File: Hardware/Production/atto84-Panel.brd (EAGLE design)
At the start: 101.1 x 104.9 mm, 1062 parts, among them U1 ATTINY84ATTINY84-20MU, U10 ATTINY84ATTINY84-20MU, U11 ATTINY84ATTINY84-20MU, U12 ATTINY84ATTINY84-20MU, U13 ATTINY84ATTINY84-20MU, U14 ATTINY84ATTINY84-20MU, U15 ATTINY84ATTINY84-20MU, U16 ATTINY84ATTINY84-20MU, U17 ATTINY84ATTINY84-20MU, U18 ATTINY84ATTINY84-20MU, U19 ATTINY84ATTINY84-20MU, U2 ATTINY84ATTINY84-20MU, U20 ATTINY84ATTINY84-20MU, U21 ATTINY84ATTINY84-20MU, U22 ATTINY84ATTINY84-20MU, U23 ATTINY84ATTINY84-20MU, U24 ATTINY84ATTINY84-20MU, U3 ATTINY84ATTINY84-20MU, U4 ATTINY84ATTINY84-20MU, U5 ATTINY84ATTINY84-20MU, U6 ATTINY84ATTINY84-20MU, U7 ATTINY84ATTINY84-20MU, U8 ATTINY84ATTINY84-20MU, U9 ATTINY84ATTINY84-20MU

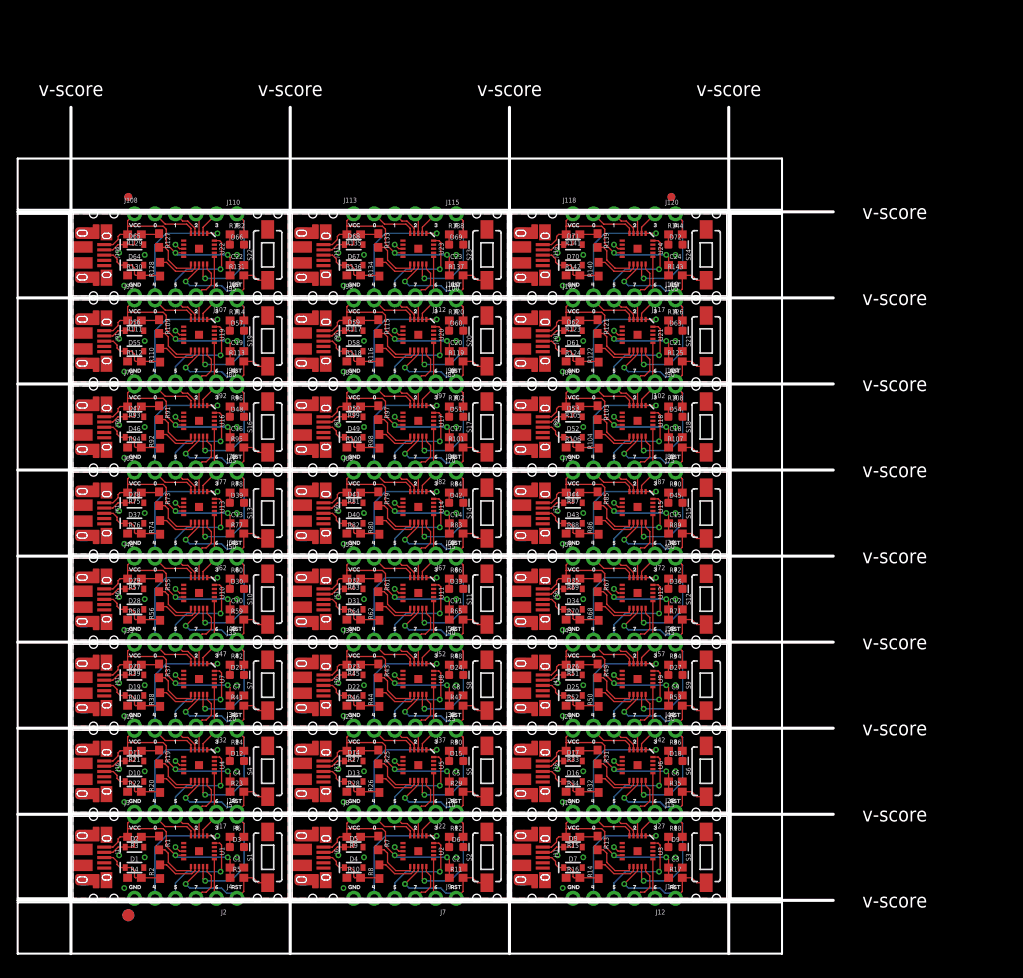
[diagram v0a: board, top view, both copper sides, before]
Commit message: Pushing "new" version
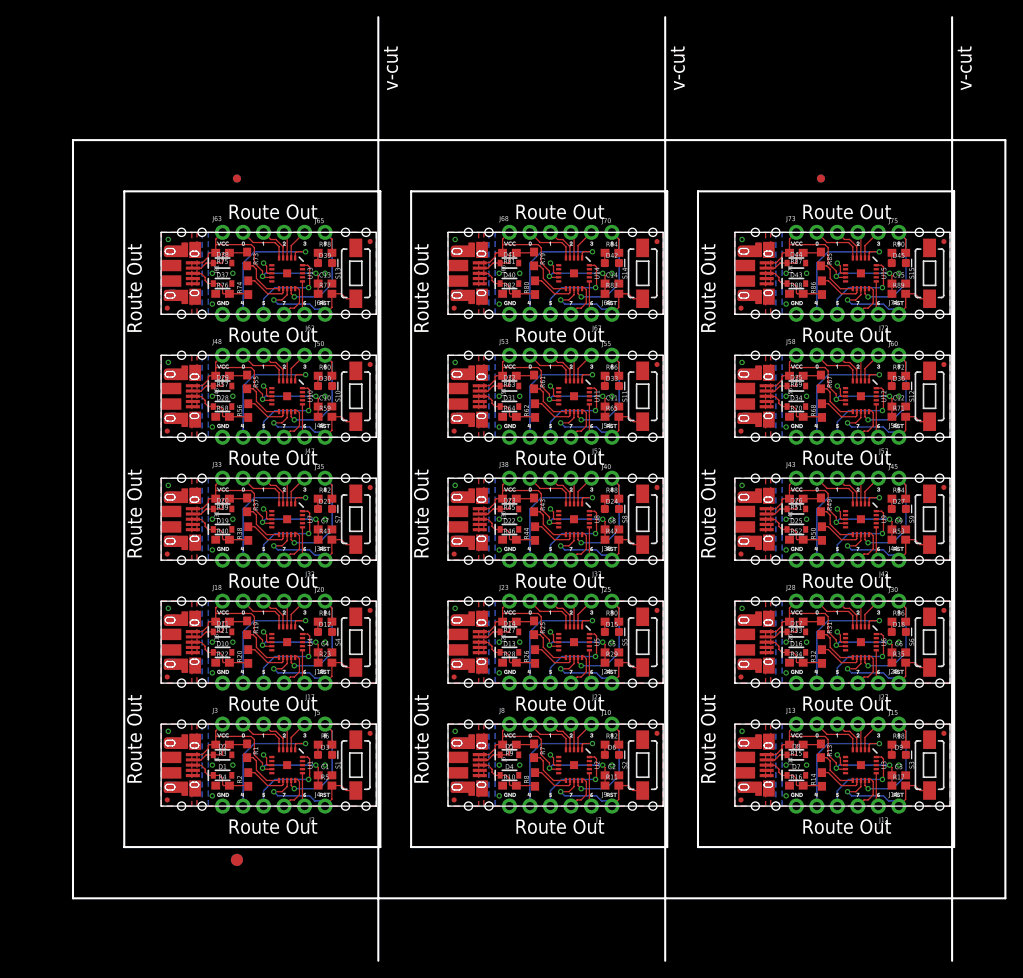
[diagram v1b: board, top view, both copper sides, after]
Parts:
- removed C16, C17, C18, C19, C20, C21, C22, C23, C24: 0.1uF, SparkFun-Capacitors:0603
- removed D46, D47, D49, D50, D52, D53, D55, D56, D58, D59, D61, D62, D64, D65, D67, D68, D70, D71: 3.6V, SparkFun-DiscreteSemi:SOD-323
- removed D48, D51, D54, D57, D60, D63, D66, D69, D72: BLUE, SparkFun-LED:LED-0603
- removed J100, J104, J105, J109, J110, J114, J115, J119, J120, J79, J80, J84, J85, J89, J90, J94, J95, J99: (no value), SparkFun-Connectors:1X01_NO_SILK
- removed J101, J106, J111, J116, J76, J81, J86, J91, J96: (no value), SparkFun-Connectors:USB-MICROB-PTH-MILL
- removed J102, J103, J107, J108, J112, J113, J117, J118, J77, J78, J82, J83, J87, J88, J92, J93, J97, J98: (no value), SparkFun-Connectors:1X05_NO_SILK
- removed R100, R106, R112, R118, R124, R130, R136, R142, R94: 1M, SparkFun-Resistors:0603
- removed R101, R107, R113, R119, R125, R131, R137, R143, R95: 10k, SparkFun-Resistors:0603
- removed R102, R108, R114, R120, R126, R132, R138, R144, R96: 1k, SparkFun-Resistors:0603
- removed R103, R104, R109, R110, R115, R116, R121, R122, R127, R128, R133, R134, R139, R140, R91, R92, R97, R98: 68OHM-0603-1/10W-1%, SparkFun-Resistors:0603
- removed R105, R111, R117, R123, R129, R135, R141, R93, R99: 1.5k, SparkFun-Resistors:0603
- removed S16, S17, S18, S19, S20, S21, S22, S23, S24: MOMENTARY-SWITCH-SPST-SMD-6.0X3.5MM, SparkFun-Switches:TACTILE_SWITCH_SMD_6.0X3.5MM
- removed U$406, U$433, U$460, U$487, U$514, U$541, U$568, U$595, U$622: (no value), buzzard_labels (20):00
- removed U$407, U$434, U$461, U$488, U$515, U$542, U$569, U$596, U$623: (no value), buzzard_labels (20):11
- removed U$408, U$435, U$462, U$489, U$516, U$543, U$570, U$597, U$624: (no value), buzzard_labels (20):22
- removed U$409, U$436, U$463, U$490, U$517, U$544, U$571, U$598, U$625: (no value), buzzard_labels (20):33
- removed U$410, U$437, U$464, U$491, U$518, U$545, U$572, U$599, U$626: (no value), buzzard_labels (20):44
- removed U$411, U$438, U$465, U$492, U$519, U$546, U$573, U$600, U$627: (no value), buzzard_labels (20):55
- removed U$412, U$439, U$466, U$493, U$520, U$547, U$574, U$601, U$628: (no value), buzzard_labels (20):66
- removed U$413, U$440, U$467, U$494, U$521, U$548, U$575, U$602, U$629: (no value), buzzard_labels (20):77
- removed U$414, U$441, U$468, U$495, U$522, U$549, U$576, U$603, U$630: (no value), buzzard_labels (20):RST8
- removed U$415, U$442, U$469, U$496, U$523, U$550, U$577, U$604, U$631: (no value), buzzard_labels (20):VCC10
- removed U$416, U$443, U$470, U$497, U$524, U$551, U$578, U$605, U$632: (no value), buzzard_labels (20):GND9
- removed U$417, U$444, U$471, U$498, U$525, U$552, U$579, U$606, U$633: (no value), buzzard_labels (21):81
- removed U$418, U$445, U$472, U$499, U$526, U$553, U$580, U$607, U$634: (no value), buzzard_labels (20):ATTO8411
- removed U$419, U$446, U$473, U$500, U$527, U$554, U$581, U$608, U$635: (no value), SparkX:SPARKX-SMALL
- removed U$420, U$447, U$474, U$501, U$528, U$555, U$582, U$609, U$636: (no value), buzzard_labels (22):VCC_5
- removed U$421, U$448, U$475, U$502, U$529, U$556, U$583, U$610, U$637: (no value), buzzard_labels (22):0_4
- removed U$422, U$449, U$476, U$503, U$530, U$557, U$584, U$611, U$638: (no value), buzzard_labels (22):1_3
- removed U$423, U$450, U$477, U$504, U$531, U$558, U$585, U$612, U$639: (no value), buzzard_labels (22):2_2
- removed U$424, U$451, U$478, U$505, U$532, U$559, U$586, U$613, U$640: (no value), buzzard_labels (22):3_1
- removed U$425, U$452, U$479, U$506, U$533, U$560, U$587, U$614, U$641: (no value), buzzard_labels (22):8_0
- removed U$426, U$453, U$480, U$507, U$534, U$561, U$588, U$615, U$642: (no value), SparkFun-Aesthetics:OSHW-LOGO-S
- removed U$427, U$454, U$481, U$508, U$535, U$562, U$589, U$616, U$643: (no value), buzzard_labels (23):_#RST0
- removed U$428, U$455, U$482, U$509, U$536, U$563, U$590, U$617, U$644: (no value), buzzard_labels (23):_42
- removed U$429, U$456, U$483, U$510, U$537, U$564, U$591, U$618, U$645: (no value), buzzard_labels (23):_53
- removed U$430, U$457, U$484, U$511, U$538, U$565, U$592, U$619, U$646: (no value), buzzard_labels (23):_64
- removed U$431, U$458, U$485, U$512, U$539, U$566, U$593, U$620, U$647: (no value), buzzard_labels (23):_75
- removed U$432, U$459, U$486, U$513, U$540, U$567, U$594, U$621, U$648: (no value), buzzard_labels (23):_GND1
- removed U16, U17, U18, U19, U20, U21, U22, U23, U24: ATTINY84ATTINY84-20MU, SparkFun-IC-Microcontroller:QFN20
- added FD1, FD10, FD11, FD12, FD13, FD14, FD15, FD16, FD17, FD18, FD19, FD2, FD20, FD21, FD22, FD23, FD24, FD25, FD26, FD27, FD28, FD29, FD3, FD30, FD4, FD5, FD6, FD7, FD8, FD9: FIDUCIALUFIDUCIAL, SparkFun-Aesthetics:FIDUCIAL-MICRO
- S1, S10, S11, S12, S13, S14, S15, S2, S3, S4, S5, S6, S7, S8, S9: value MOMENTARY-SWITCH-SPST-SMD-6.0X3.5MM -> (none)
- moved J71 41.6 mm to (86.0, 77.5)
- moved D43 40.6 mm to (89.7, 76.2)
- moved D44 40.6 mm to (89.7, 78.7)
- moved J72 40.6 mm to (99.8, 72.4)
- moved J73 40.6 mm to (89.7, 82.5)
- moved R86 40.6 mm to (92.8, 75.7)
- moved R87 40.6 mm to (89.7, 80.0)
- moved R88 40.6 mm to (89.7, 74.9)
- moved U$381 40.6 mm to (96.6, 81.2)
- moved U$386 40.6 mm to (96.6, 73.8)
- moved U$388 40.6 mm to (88.5, 81.2)
- moved U$389 40.6 mm to (88.5, 73.8)
- moved U$390 40.6 mm to (101.7, 81.2)
- moved U$393 40.6 mm to (89.7, 77.5)
- moved U$395 40.6 mm to (94.7, 79.6)
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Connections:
- removed net !RESET15: J79.1, R95.2, S16.1, U16.13
- removed net !RESET16: J84.1, R101.2, S17.1, U17.13
- removed net !RESET17: J89.1, R107.2, S18.1, U18.13
- removed net !RESET18: J94.1, R113.2, S19.1, U19.13
- removed net !RESET19: J99.1, R119.2, S20.1, U20.13
- removed net !RESET20: J104.1, R125.2, S21.1, U21.13
- removed net !RESET21: J109.1, R131.2, S22.1, U22.13
- removed net !RESET22: J114.1, R137.2, S23.1, U23.13
- removed net !RESET23: J119.1, R143.2, S24.1, U24.13
- removed net D+15: D46.C, J76.D+, R92.1, R94.2
- removed net D+16: D49.C, J81.D+, R100.2, R98.1
- removed net D+17: D52.C, J86.D+, R104.1, R106.2
- removed net D+18: D55.C, J91.D+, R110.1, R112.2
- removed net D+19: D58.C, J96.D+, R116.1, R118.2
- removed net D+20: D61.C, J101.D+, R122.1, R124.2
- removed net D+21: D64.C, J106.D+, R128.1, R130.2
- removed net D+22: D67.C, J111.D+, R134.1, R136.2
- removed net D+23: D70.C, J116.D+, R140.1, R142.2
- removed net D-15: D47.C, J76.D-, R91.1, R93.1
- removed net D-16: D50.C, J81.D-, R97.1, R99.1
- removed net D-17: D53.C, J86.D-, R103.1, R105.1
- removed net D-18: D56.C, J91.D-, R109.1, R111.1
- removed net D-19: D59.C, J96.D-, R115.1, R117.1
- removed net D-20: D62.C, J101.D-, R121.1, R123.1
- removed net D-21: D65.C, J106.D-, R127.1, R129.1
- removed net D-22: D68.C, J111.D-, R133.1, R135.1
- removed net D-23: D71.C, J116.D-, R139.1, R141.1
- removed net D120: J78.2, U16.5
- removed net D121: J78.3, U16.4
- removed net D122: J78.4, U16.3
- removed net D123: J78.5, U16.2
- removed net D124: J77.4, U16.1
- removed net D125: J77.3, U16.20
- removed net D126: J77.1, U16.16
- removed net D127: J77.2, U16.15
- removed net D128: J83.2, U17.5
- removed net D129: J83.3, U17.4
- removed net D130: J83.4, U17.3
- removed net D131: J83.5, U17.2
- removed net D132: J82.4, U17.1
- removed net D133: J82.3, U17.20
- removed net D134: J82.1, U17.16
- removed net D135: J82.2, U17.15
- removed net D136: J88.2, U18.5
- removed net D137: J88.3, U18.4
- removed net D138: J88.4, U18.3
- removed net D139: J88.5, U18.2
- removed net D140: J87.4, U18.1
- removed net D141: J87.3, U18.20
- removed net D142: J87.1, U18.16
- removed net D143: J87.2, U18.15
- removed net D144: J93.2, U19.5
- removed net D145: J93.3, U19.4
- removed net D146: J93.4, U19.3
- removed net D147: J93.5, U19.2
- removed net D148: J92.4, U19.1
- removed net D149: J92.3, U19.20
- removed net D150: J92.1, U19.16
- removed net D151: J92.2, U19.15
- removed net D152: J98.2, U20.5
- removed net D153: J98.3, U20.4
- removed net D154: J98.4, U20.3
- removed net D155: J98.5, U20.2
- removed net D156: J97.4, U20.1
- removed net D157: J97.3, U20.20
- removed net D158: J97.1, U20.16
- removed net D159: J97.2, U20.15
- removed net D160: J103.2, U21.5
- removed net D161: J103.3, U21.4
- removed net D162: J103.4, U21.3
- removed net D163: J103.5, U21.2
- removed net D164: J102.4, U21.1
- removed net D165: J102.3, U21.20
- removed net D166: J102.1, U21.16
- removed net D167: J102.2, U21.15
- removed net D168: J108.2, U22.5
- removed net D169: J108.3, U22.4
- removed net D170: J108.4, U22.3
- removed net D171: J108.5, U22.2
- removed net D172: J107.4, U22.1
- removed net D173: J107.3, U22.20
- removed net D174: J107.1, U22.16
- removed net D175: J107.2, U22.15
- removed net D176: J113.2, U23.5
- removed net D177: J113.3, U23.4
- removed net D178: J113.4, U23.3
- removed net D179: J113.5, U23.2
- removed net D180: J112.4, U23.1
- removed net D181: J112.3, U23.20
- removed net D182: J112.1, U23.16
- removed net D183: J112.2, U23.15
- removed net D184: J118.2, U24.5
- removed net D185: J118.3, U24.4
- removed net D186: J118.4, U24.3
- removed net D187: J118.5, U24.2
- removed net D188: J117.4, U24.1
- removed net D189: J117.3, U24.20
- removed net D190: J117.1, U24.16
- removed net D191: J117.2, U24.15
- removed net GND15: C16.2, D46.A, D47.A, D48.C, J76.GND, J77.5, R94.1, S16.2, U16.8
- removed net GND16: C17.2, D49.A, D50.A, D51.C, J81.GND, J82.5, R100.1, S17.2, U17.8
- removed net GND17: C18.2, D52.A, D53.A, D54.C, J86.GND, J87.5, R106.1, S18.2, U18.8
- removed net GND18: C19.2, D55.A, D56.A, D57.C, J91.GND, J92.5, R112.1, S19.2, U19.8
- removed net GND19: C20.2, D58.A, D59.A, D60.C, J96.GND, J97.5, R118.1, S20.2, U20.8
- removed net GND20: C21.2, D61.A, D62.A, D63.C, J101.GND, J102.5, R124.1, S21.2, U21.8
- removed net GND21: C22.2, D64.A, D65.A, D66.C, J106.GND, J107.5, R130.1, S22.2, U22.8
- removed net GND22: C23.2, D67.A, D68.A, D69.C, J111.GND, J112.5, R136.1, S23.2, U23.8
- removed net GND23: C24.2, D70.A, D71.A, D72.C, J116.GND, J117.5, R142.1, S24.2, U24.8
- removed net N$16: D48.A, R96.1
- removed net N$17: D51.A, R102.1
- removed net N$18: D54.A, R108.1
- removed net N$19: D57.A, R114.1
- removed net N$20: D60.A, R120.1
- removed net N$21: D63.A, R126.1
- removed net N$22: D66.A, R132.1
- removed net N$23: D69.A, R138.1
- removed net N$24: D72.A, R144.1
- removed net PB30: R91.2, U16.11
- removed net PB31: R92.2, U16.12
- removed net PB32: R97.2, U17.11
- removed net PB33: R98.2, U17.12
- removed net PB34: R103.2, U18.11
- removed net PB35: R104.2, U18.12
- removed net PB36: R109.2, U19.11
- removed net PB37: R110.2, U19.12
- removed net PB38: R115.2, U20.11
- removed net PB39: R116.2, U20.12
- removed net PB40: R121.2, U21.11
- removed net PB41: R122.2, U21.12
- removed net PB42: R127.2, U22.11
- removed net PB43: R128.2, U22.12
- removed net PB44: R133.2, U23.11
- removed net PB45: R134.2, U23.12
- removed net PB46: R139.2, U24.11
- removed net PB47: R140.2, U24.12
- removed net STATUS15: J80.1, R96.2, U16.14
- removed net STATUS16: J85.1, R102.2, U17.14
- removed net STATUS17: J90.1, R108.2, U18.14
- removed net STATUS18: J95.1, R114.2, U19.14
- removed net STATUS19: J100.1, R120.2, U20.14
- removed net STATUS20: J105.1, R126.2, U21.14
- removed net STATUS21: J110.1, R132.2, U22.14
- removed net STATUS22: J115.1, R138.2, U23.14
- removed net STATUS23: J120.1, R144.2, U24.14
- removed net VCC15: C16.1, J76.VBUS, J78.1, R93.2, R95.1, U16.9
- removed net VCC16: C17.1, J81.VBUS, J83.1, R101.1, R99.2, U17.9
- removed net VCC17: C18.1, J86.VBUS, J88.1, R105.2, R107.1, U18.9
- removed net VCC18: C19.1, J91.VBUS, J93.1, R111.2, R113.1, U19.9
- removed net VCC19: C20.1, J96.VBUS, J98.1, R117.2, R119.1, U20.9
- removed net VCC20: C21.1, J101.VBUS, J103.1, R123.2, R125.1, U21.9
- removed net VCC21: C22.1, J106.VBUS, J108.1, R129.2, R131.1, U22.9
- removed net VCC22: C23.1, J111.VBUS, J113.1, R135.2, R137.1, U23.9
- removed net VCC23: C24.1, J116.VBUS, J118.1, R141.2, R143.1, U24.9
- new net SHLD: J1.SHIELD, J1.SHIELD10, J1.SHIELD2, J1.SHIELD3, J1.SHIELD4, J1.SHIELD5, J1.SHIELD6, J1.SHIELD7, J1.SHIELD8, J1.SHIELD9
- new net SHLD1: J6.SHIELD, J6.SHIELD10, J6.SHIELD2, J6.SHIELD3, J6.SHIELD4, J6.SHIELD5, J6.SHIELD6, J6.SHIELD7, J6.SHIELD8, J6.SHIELD9
- new net SHLD10: J51.SHIELD, J51.SHIELD10, J51.SHIELD2, J51.SHIELD3, J51.SHIELD4, J51.SHIELD5, J51.SHIELD6, J51.SHIELD7, J51.SHIELD8, J51.SHIELD9
- new net SHLD11: J56.SHIELD, J56.SHIELD10, J56.SHIELD2, J56.SHIELD3, J56.SHIELD4, J56.SHIELD5, J56.SHIELD6, J56.SHIELD7, J56.SHIELD8, J56.SHIELD9
- new net SHLD12: J61.SHIELD, J61.SHIELD10, J61.SHIELD2, J61.SHIELD3, J61.SHIELD4, J61.SHIELD5, J61.SHIELD6, J61.SHIELD7, J61.SHIELD8, J61.SHIELD9
- new net SHLD13: J66.SHIELD, J66.SHIELD10, J66.SHIELD2, J66.SHIELD3, J66.SHIELD4, J66.SHIELD5, J66.SHIELD6, J66.SHIELD7, J66.SHIELD8, J66.SHIELD9
- new net SHLD14: J71.SHIELD, J71.SHIELD10, J71.SHIELD2, J71.SHIELD3, J71.SHIELD4, J71.SHIELD5, J71.SHIELD6, J71.SHIELD7, J71.SHIELD8, J71.SHIELD9
- new net SHLD2: J11.SHIELD, J11.SHIELD10, J11.SHIELD2, J11.SHIELD3, J11.SHIELD4, J11.SHIELD5, J11.SHIELD6, J11.SHIELD7, J11.SHIELD8, J11.SHIELD9
- new net SHLD3: J16.SHIELD, J16.SHIELD10, J16.SHIELD2, J16.SHIELD3, J16.SHIELD4, J16.SHIELD5, J16.SHIELD6, J16.SHIELD7, J16.SHIELD8, J16.SHIELD9
- new net SHLD4: J21.SHIELD, J21.SHIELD10, J21.SHIELD2, J21.SHIELD3, J21.SHIELD4, J21.SHIELD5, J21.SHIELD6, J21.SHIELD7, J21.SHIELD8, J21.SHIELD9
- new net SHLD5: J26.SHIELD, J26.SHIELD10, J26.SHIELD2, J26.SHIELD3, J26.SHIELD4, J26.SHIELD5, J26.SHIELD6, J26.SHIELD7, J26.SHIELD8, J26.SHIELD9
- new net SHLD6: J31.SHIELD, J31.SHIELD10, J31.SHIELD2, J31.SHIELD3, J31.SHIELD4, J31.SHIELD5, J31.SHIELD6, J31.SHIELD7, J31.SHIELD8, J31.SHIELD9
- new net SHLD7: J36.SHIELD, J36.SHIELD10, J36.SHIELD2, J36.SHIELD3, J36.SHIELD4, J36.SHIELD5, J36.SHIELD6, J36.SHIELD7, J36.SHIELD8, J36.SHIELD9
- new net SHLD8: J41.SHIELD, J41.SHIELD10, J41.SHIELD2, J41.SHIELD3, J41.SHIELD4, J41.SHIELD5, J41.SHIELD6, J41.SHIELD7, J41.SHIELD8, J41.SHIELD9
- new net SHLD9: J46.SHIELD, J46.SHIELD10, J46.SHIELD2, J46.SHIELD3, J46.SHIELD4, J46.SHIELD5, J46.SHIELD6, J46.SHIELD7, J46.SHIELD8, J46.SHIELD9
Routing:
- net VCC19: track 25.1 -> 0.00 mm, vias 2 -> 0
- net VCC22: track 25.1 -> 0.00 mm, vias 2 -> 0
- net VCC18: track 25.1 -> 0.00 mm, vias 2 -> 0
- net VCC16: track 25.1 -> 0.00 mm, vias 2 -> 0
- net VCC15: track 25.1 -> 0.00 mm, vias 2 -> 0
- net VCC21: track 25.1 -> 0.00 mm, vias 2 -> 0
- net VCC23: track 25.1 -> 0.00 mm, vias 2 -> 0
- net VCC20: track 25.1 -> 0.00 mm, vias 2 -> 0
- net VCC17: track 25.1 -> 0.00 mm, vias 2 -> 0
- net STATUS19: track 17.0 -> 0.00 mm, vias 1 -> 0
- net STATUS18: track 17.0 -> 0.00 mm, vias 1 -> 0
- net STATUS22: track 17.0 -> 0.00 mm, vias 1 -> 0
- net STATUS21: track 17.0 -> 0.00 mm, vias 1 -> 0
- net STATUS20: track 17.0 -> 0.00 mm, vias 1 -> 0
- net STATUS16: track 17.0 -> 0.00 mm, vias 1 -> 0
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- added copper zone on layer 1, net SHLD
- added copper zone on layer 16, net SHLD
- added copper zone on layer 1, net SHLD1
- added copper zone on layer 16, net SHLD1
- added copper zone on layer 1, net SHLD10
- added copper zone on layer 16, net SHLD10
- added copper zone on layer 1, net SHLD11
- added copper zone on layer 16, net SHLD11
- added copper zone on layer 1, net SHLD12
- added copper zone on layer 16, net SHLD12
- added copper zone on layer 1, net SHLD13
- added copper zone on layer 16, net SHLD13
- added copper zone on layer 1, net SHLD14
- added copper zone on layer 16, net SHLD14
- added copper zone on layer 1, net SHLD2
- added copper zone on layer 16, net SHLD2
- added copper zone on layer 1, net SHLD3
- added copper zone on layer 16, net SHLD3
- added copper zone on layer 1, net SHLD4
- added copper zone on layer 16, net SHLD4
- added copper zone on layer 1, net SHLD5
- added copper zone on layer 16, net SHLD5
- added copper zone on layer 1, net SHLD6
- added copper zone on layer 16, net SHLD6
- added copper zone on layer 1, net SHLD7
- added copper zone on layer 16, net SHLD7
- added copper zone on layer 1, net SHLD8
- added copper zone on layer 16, net SHLD8
- added copper zone on layer 1, net SHLD9
- added copper zone on layer 16, net SHLD9
- removed copper zone on layer 1, net GND15
- removed copper zone on layer 16, net GND15
- removed copper zone on layer 1, net GND16
- removed copper zone on layer 16, net GND16
- removed copper zone on layer 1, net GND17
- removed copper zone on layer 16, net GND17
- removed copper zone on layer 1, net GND18
- removed copper zone on layer 16, net GND18
- removed copper zone on layer 1, net GND19
- removed copper zone on layer 16, net GND19
- removed copper zone on layer 1, net GND20
- removed copper zone on layer 16, net GND20
- removed copper zone on layer 1, net GND21
- removed copper zone on layer 16, net GND21
- removed copper zone on layer 1, net GND22
- removed copper zone on layer 16, net GND22
- removed copper zone on layer 1, net GND23
- removed copper zone on layer 16, net GND23
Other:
- board size 101.1 x 104.9 mm -> 115.6 x 117 mm
- board text added: "Route Out"
- board text added: "v-cut"
- board text removed: "v-score"
